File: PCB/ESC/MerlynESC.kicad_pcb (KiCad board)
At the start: 6 copper layers, 30.5 x 31.9 mm, 155 parts, among them M1 BLDC Motor, M2 BLDC Motor, M3 BLDC Motor, M4 BLDC Motor, Q1 JMSL0302AU, Q10 JMSL0302AU, Q11 JMSL0302AU, Q12 JMSL0302AU, Q13 JMSL0302AU, Q14 JMSL0302AU, Q15 JMSL0302AU, Q16 JMSL0302AU, Q17 JMSL0302AU, Q18 JMSL0302AU, Q19 JMSL0302AU, Q2 JMSL0302AU, Q20 JMSL0302AU, Q21 JMSL0302AU, Q22 JMSL0302AU, Q23 JMSL0302AU, Q24 JMSL0302AU, Q3 JMSL0302AU, Q4 JMSL0302AU, Q5 JMSL0302AU, Q6 JMSL0302AU, Q7 JMSL0302AU, Q8 JMSL0302AU, Q9 JMSL0302AU, U1 HT75C0-1, U10 EG6288, U11 EFM8BB21F16G, U2 HT7533-1, U3 EFM8BB21F16G, U4 EG6288, U5 EG6288, U6 EFM8BB21F16G, U7 INA139NA, U8 EG6288, U9 EFM8BB21F16G

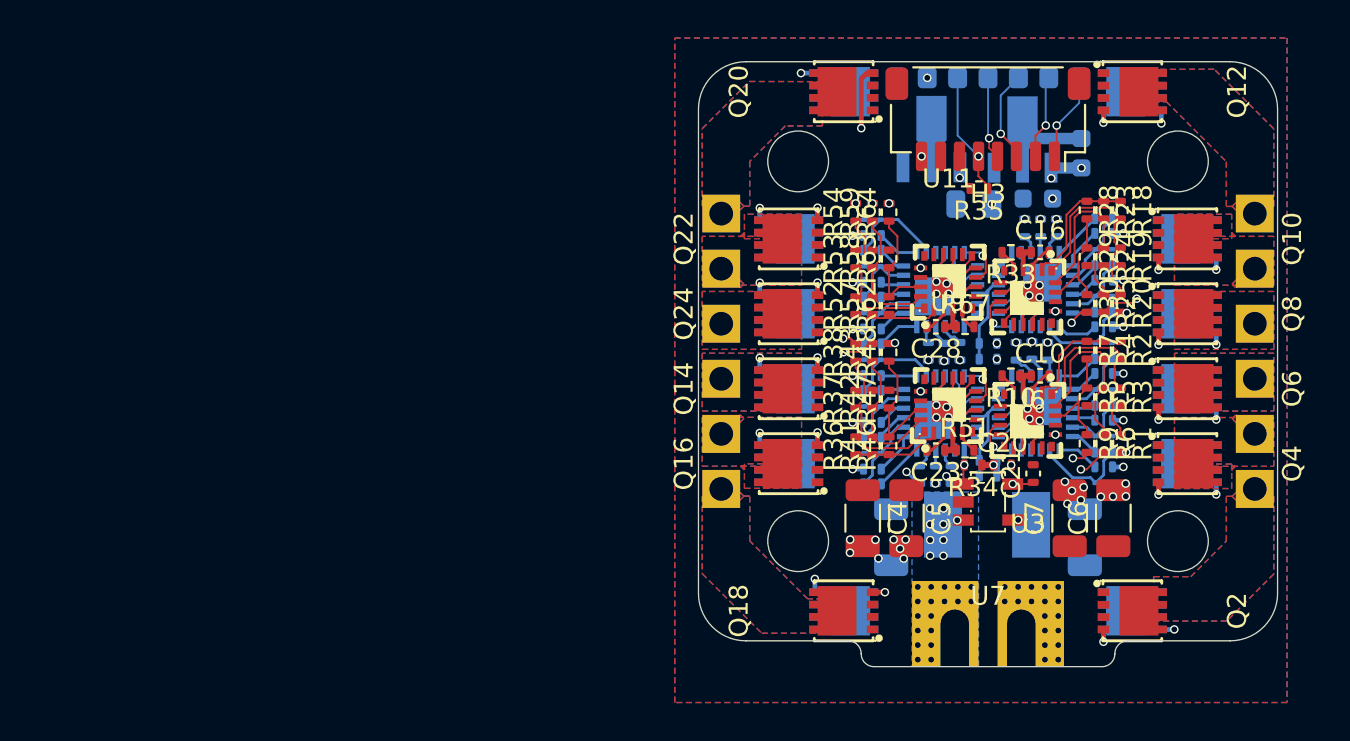
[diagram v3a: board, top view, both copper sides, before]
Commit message: checkpoint
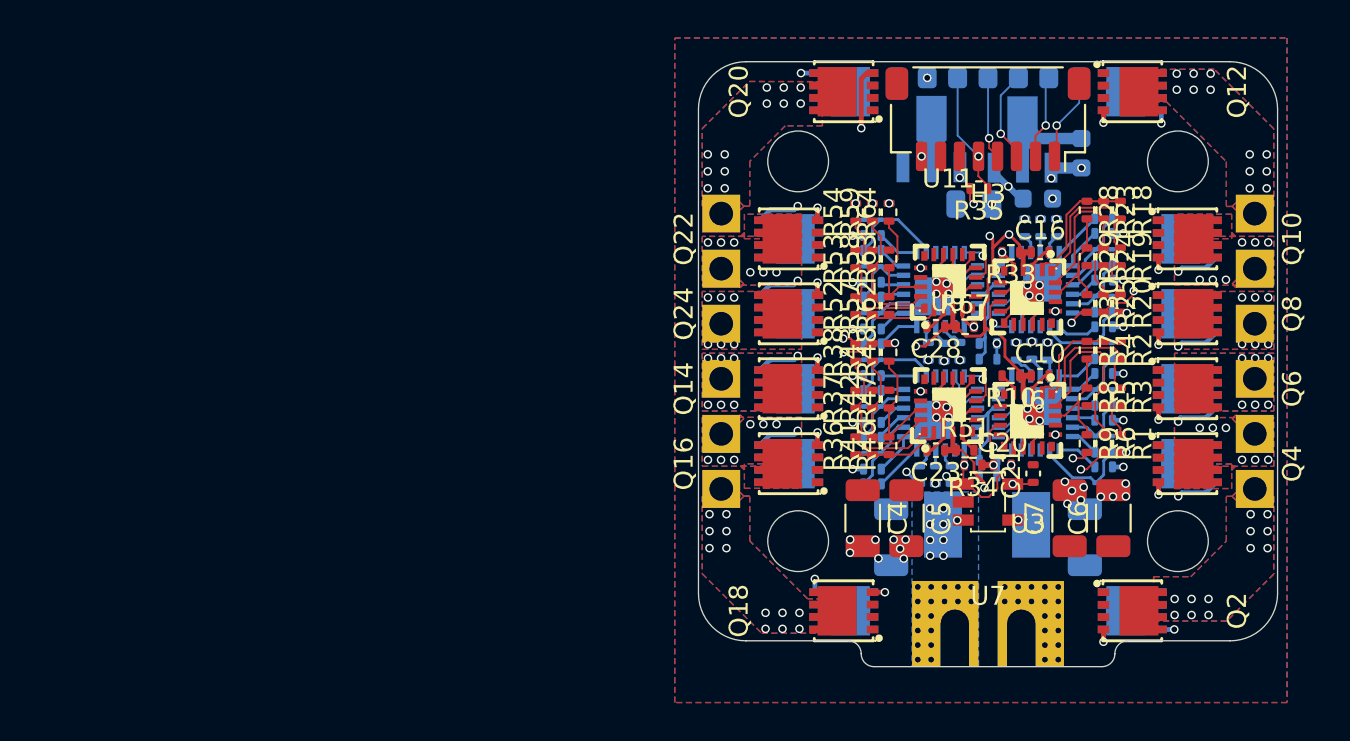
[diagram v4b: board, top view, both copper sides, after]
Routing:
- net +3.3V: track 6.34 -> 43.1 mm, vias 0 -> 5
- net Net-(U7-OUT): track 1.02 -> 20.0 mm, vias 2 -> 3
- net M2_PHASE1: track 3.57 -> 7.31 mm, vias 1 -> 7
- net M3_PHASE1: track 6.13 -> 9.67 mm, vias 1 -> 7
- net M1_PHASE3: track 7.54 -> 11.0 mm, vias 1 -> 7
- net M4_PHASE3: track 7.36 -> 10.8 mm, vias 1 -> 7
- net Net-(Q11-G): track 7.83 -> 9.98 mm
- net M1_PHASE1: track 7.25 -> 9.38 mm, vias 1 -> 13
- net M2_PHASE2: track 4.55 -> 5.87 mm, vias 1 -> 7
- net M3_PHASE2: track 6.74 -> 8.00 mm, vias 1 -> 7
- net Net-(Q3-G): track 7.72 -> 8.79 mm
- net M1_PHASE2: track 8.05 -> 9.08 mm, vias 1 -> 7
- net GND: track 14.9 -> 15.7 mm, vias 43 -> 42
- net M4_PHASE2: track 6.63 -> 7.44 mm, vias 1 -> 7
- net Net-(Q4-G): track 12.7 -> 13.5 mm
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- removed copper zone on In1.Cu, net M1_PHASE1
- removed copper zone on In2.Cu, net M1_PHASE1
- removed copper zone on In3.Cu, net M1_PHASE1
- removed copper zone on In4.Cu, net M1_PHASE1
- removed copper zone on In1.Cu, net M1_PHASE2
- removed copper zone on In2.Cu, net M1_PHASE2
- removed copper zone on In3.Cu, net M1_PHASE2
- removed copper zone on In4.Cu, net M1_PHASE2
- removed copper zone on In1.Cu, net M1_PHASE3
- removed copper zone on In2.Cu, net M1_PHASE3
- removed copper zone on In3.Cu, net M1_PHASE3
- removed copper zone on In4.Cu, net M1_PHASE3
- removed copper zone on In1.Cu, net M2_PHASE1
- removed copper zone on In2.Cu, net M2_PHASE1
- removed copper zone on In3.Cu, net M2_PHASE1
- removed copper zone on In4.Cu, net M2_PHASE1
- removed copper zone on In1.Cu, net M2_PHASE2
- removed copper zone on In2.Cu, net M2_PHASE2
- removed copper zone on In3.Cu, net M2_PHASE2
- removed copper zone on In4.Cu, net M2_PHASE2
- removed copper zone on In1.Cu, net M2_PHASE3
- removed copper zone on In2.Cu, net M2_PHASE3
- removed copper zone on In3.Cu, net M2_PHASE3
- removed copper zone on In4.Cu, net M2_PHASE3
- removed copper zone on In1.Cu, net M3_PHASE1
- removed copper zone on In2.Cu, net M3_PHASE1
- removed copper zone on In3.Cu, net M3_PHASE1
- removed copper zone on In4.Cu, net M3_PHASE1
- removed copper zone on In1.Cu, net M3_PHASE2
- removed copper zone on In2.Cu, net M3_PHASE2
- removed copper zone on In3.Cu, net M3_PHASE2
- removed copper zone on In4.Cu, net M3_PHASE2
- removed copper zone on In1.Cu, net M3_PHASE3
- removed copper zone on In2.Cu, net M3_PHASE3
- removed copper zone on In3.Cu, net M3_PHASE3
- removed copper zone on In4.Cu, net M3_PHASE3
- removed copper zone on In1.Cu, net M4_PHASE1
- removed copper zone on In2.Cu, net M4_PHASE1
- removed copper zone on In3.Cu, net M4_PHASE1
- removed copper zone on In4.Cu, net M4_PHASE1
- removed copper zone on In1.Cu, net M4_PHASE2
- removed copper zone on In2.Cu, net M4_PHASE2
- removed copper zone on In3.Cu, net M4_PHASE2
- removed copper zone on In4.Cu, net M4_PHASE2
- removed copper zone on In1.Cu, net M4_PHASE3
- removed copper zone on In2.Cu, net M4_PHASE3
- removed copper zone on In3.Cu, net M4_PHASE3
- removed copper zone on In4.Cu, net M4_PHASE3
